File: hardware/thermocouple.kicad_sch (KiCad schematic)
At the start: 3 parts, among them U4 MAX6675

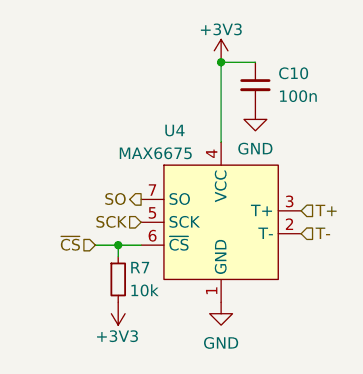
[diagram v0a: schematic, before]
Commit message: finished layout
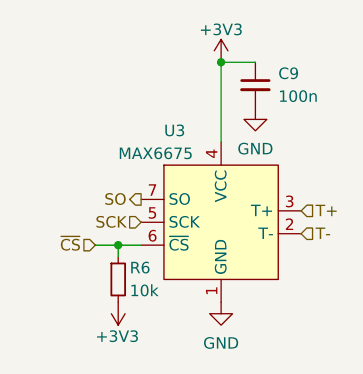
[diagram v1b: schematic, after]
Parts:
- renumbered C10 to C9, R7 to R6, U4 to U3
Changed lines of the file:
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@@
   (symbol (lib_id "Device:R_Small") (at 137.16 107.95 0)
     (in_bom yes) (on_board yes)
-    (property "Reference" "R7" (id 0) (at 138.43 106.68 0)
+    (property "Reference" "R6" (id 0) (at 138.43 106.68 0)
       (effects (font (size 1.27 1.27)) (justify left))
     )
@@
   (symbol (lib_id "extraparts:MAX6675") (at 148.59 101.6 0)
     (in_bom yes) (on_board yes)
-    (property "Reference" "U4" (id 0) (at 142.24 91.44 0)
+    (property "Reference" "U3" (id 0) (at 142.24 91.44 0)
       (effects (font (size 1.27 1.27)) (justify left))
     )
@@
   (symbol (lib_id "Device:C_Small") (at 152.4 86.36 0)
     (in_bom yes) (on_board yes)
-    (property "Reference" "C10" (id 0) (at 154.94 85.09 0)
+    (property "Reference" "C9" (id 0) (at 154.94 85.09 0)
       (effects (font (size 1.27 1.27)) (justify left))
     )
